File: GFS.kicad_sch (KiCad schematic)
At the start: 45 parts

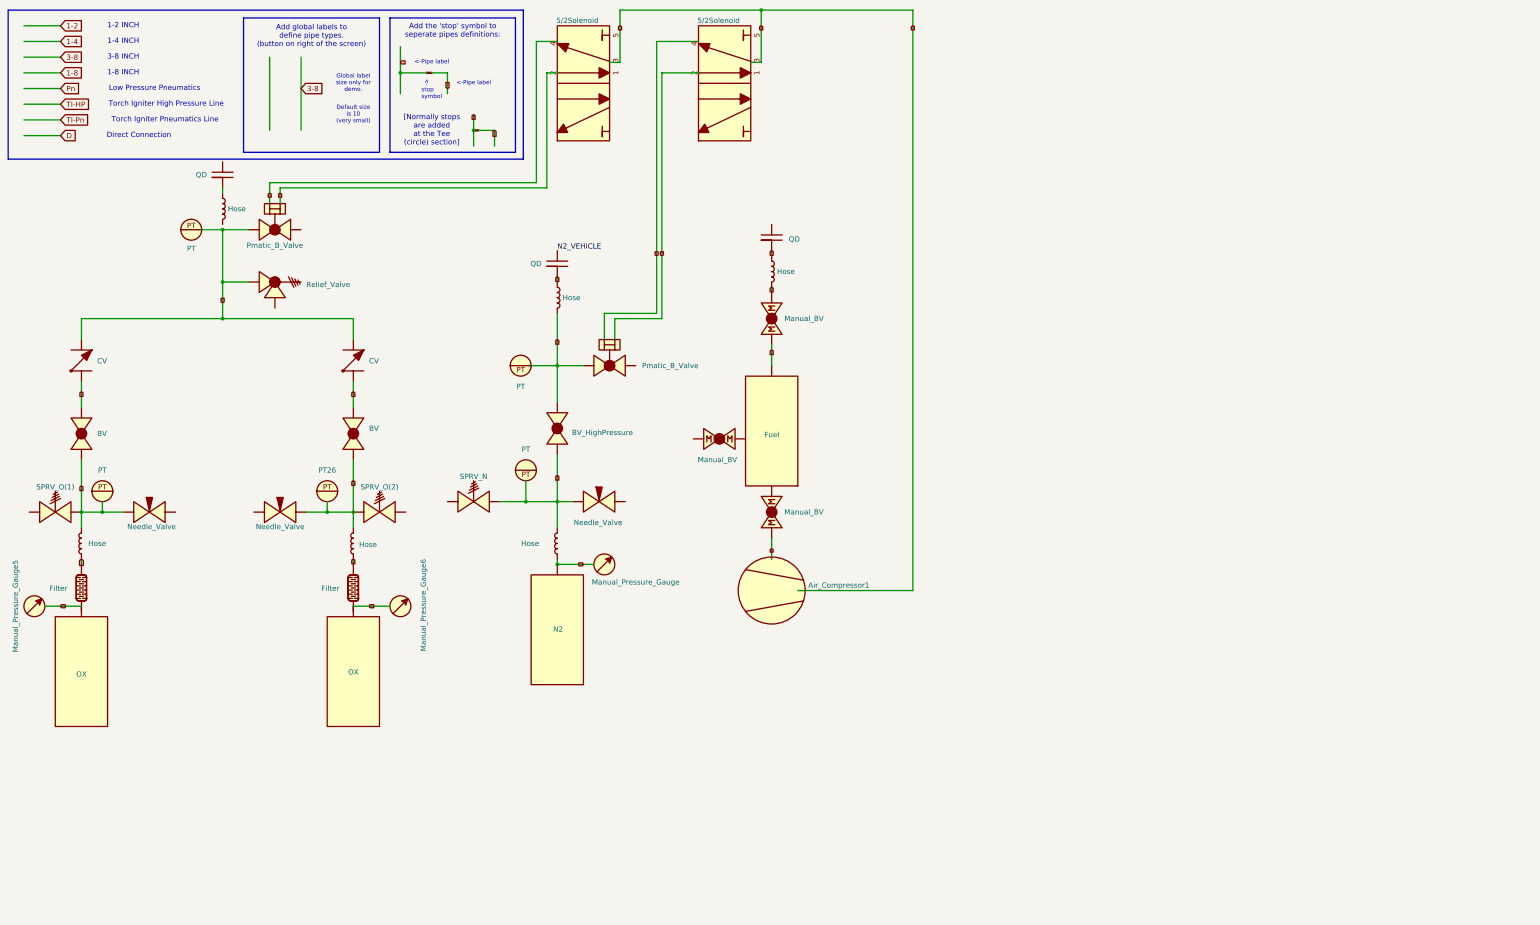
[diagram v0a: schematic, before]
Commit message: clean pnid
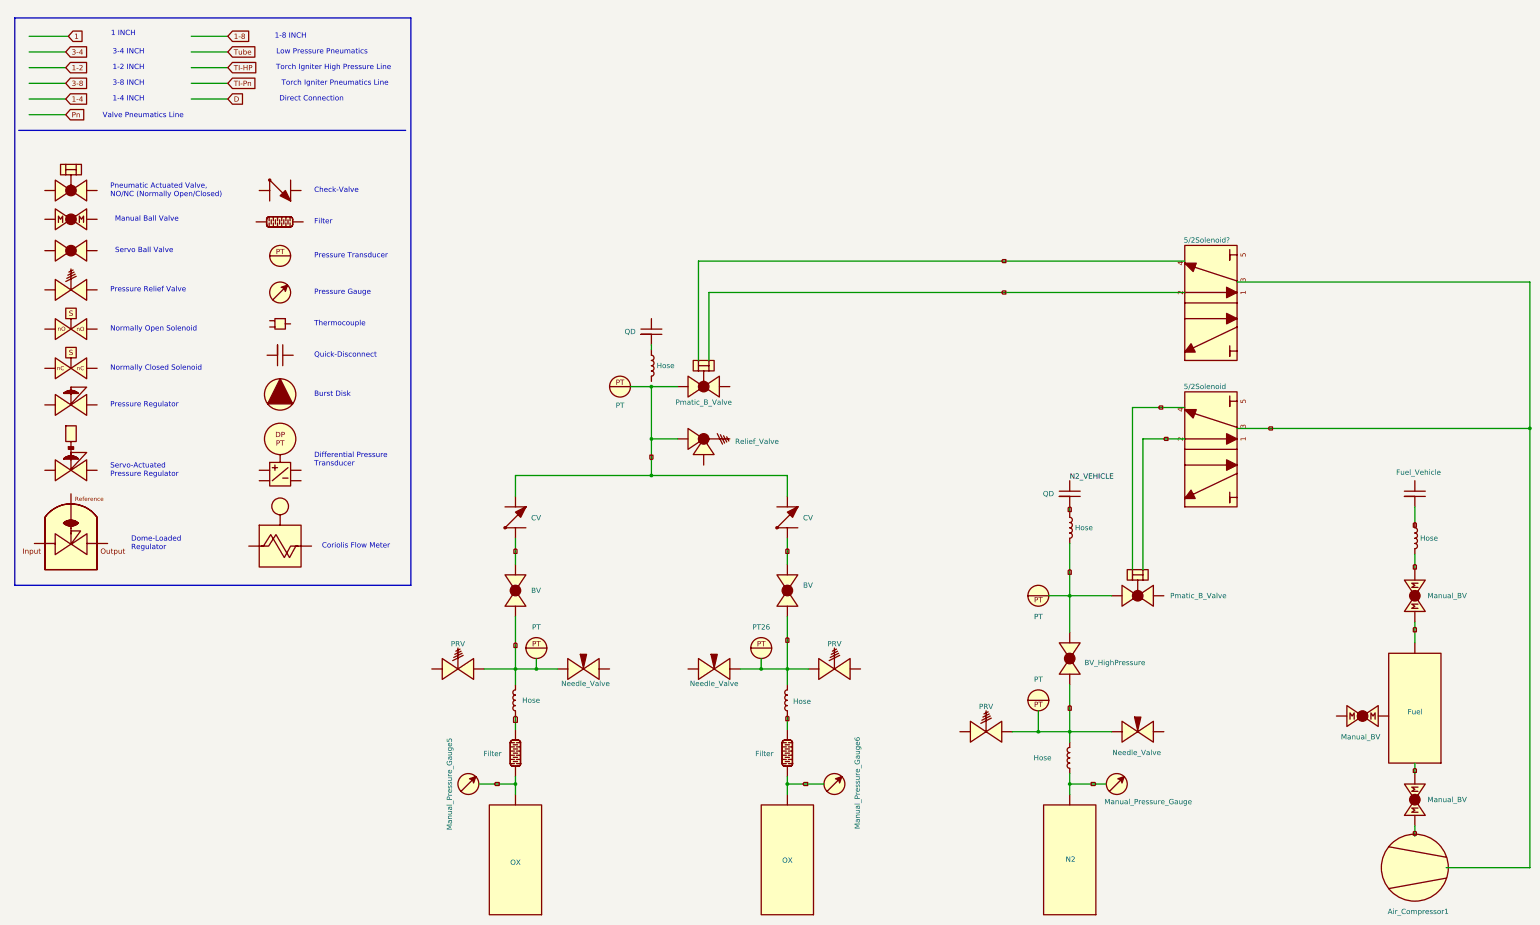
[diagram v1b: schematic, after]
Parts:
- removed 5/2Solenoid: ~, symbol PID_symbols:Solenoid_5/2
- removed U25, U26: ~, symbol PID_symbols:stop
- added BV46: ~, symbol PID_symbols:Ball_Valve
- added Burst_Disc24: ~, symbol PID_symbols:Burst_Disc
- added CF9: ~, symbol PID_symbols:Coriolis_Flow
- added CV17: ~, symbol PID_symbols:Check_Valve
- added DP9: ~, symbol PID_symbols:DP_Sensor
- added Dome9: ~, symbol PID_symbols:Dome_Reg
- added Filter4: ~, symbol PID_symbols:Filter
- added MB_V20: ~, symbol PID_symbols:MBallValve
- added Manual_Pressure_Gauge27: ~, symbol PID_symbols:Manual_Pressure_Gauge
- added PT25: ~, symbol PID_symbols:Pressure_Transducer
- added Pmatic_B_Valve18: ~, symbol PID_symbols:Pneumatic_Rotary_Ball_Valve
- added QD31: ~, symbol PID_symbols:Quick_Disconnect
- added SPRV12: ~, symbol PID_symbols:SPRV
- added Servo_Reg10, Servo_Reg24: ~, symbol PID_symbols:Pressure_Regulator
- added TC16: ~, symbol PID_symbols:Thermocouple
- added nC_Sol15: ~, symbol PID_symbols:Normally_Closed_Solenoid
- added nO_Sol33: ~, symbol PID_symbols:Normally Open Solenoid
- renumbered QD to Fuel_Vehicle, SPRV_O(1) to PRV, SPRV_N to PRV, SPRV_O(2) to PRV
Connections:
- net D: no longer Manual_BV.
- net Pn: now also Manual_BV.
- net at QD.: now also Hose.
- net at Hose.: no longer QD.
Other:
- note added: "1 INCH"
- note added: "3-4 INCH"
- note added: "Burst Disk"
- note added: "Check-Valve"
- note added: "Coriolis Flow Meter"
- note added: "Differential Pressure Transducer"
- note added: "Dome-Loaded Regulator"
- note added: "Filter"
- note added: "Manual Ball Valve"
- note added: "Normally Closed Solenoid"
- note added: "Normally Open Solenoid"
- note added: "Pneumatic Actuated Valve, NO/NC (Normally Open/Closed)"
- note added: "Pressure Gauge"
- note added: "Pressure Regulator"
- note added: "Pressure Relief Valve"
- note added: "Pressure Transducer"
- note added: "Quick-Disconnect"
- note added: "Servo Ball Valve"
- note added: "Servo-Actuated Pressure Regulator"
- note added: "Thermocouple"
- note added: "Valve Pneumatics Line"
- note removed: "->"
- note removed: "<-Pipe label"
- note removed: "Add global labels to define pipe types. (button on right of the screen)"
- note removed: "Add the 'stop' symbol to seperate pipes definitions:"
- note removed: "Default size is 10 (very small)"
- note removed: "Global label size only for demo."
- note removed: "[Normally stops are added at the Tee (circle) section]"
- note removed: "stop symbol"
- moved on the sheet: 5/2Solenoid?, Air_Compressor1, BV, BV_HighPressure, CV, Filter, Fuel, Fuel_Vehicle, Hose, Manual_BV, Manual_Pressure_Gauge, Manual_Pressure_Gauge5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
